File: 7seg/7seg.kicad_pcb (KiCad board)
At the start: 2 copper layers, 58 x 88 mm, 37 parts, among them J1 Conn_01x07, J2 Conn_01x06, J3 Conn_01x07, J4 Conn_01x06

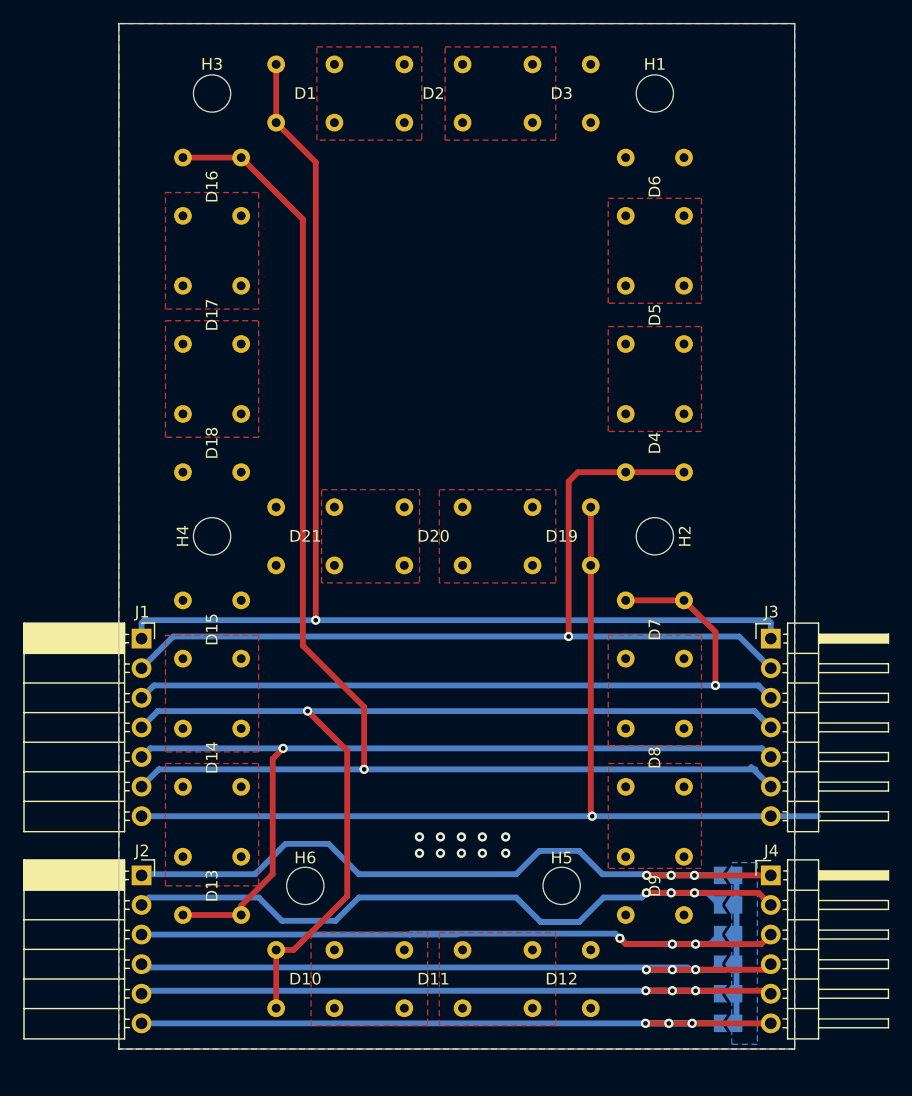
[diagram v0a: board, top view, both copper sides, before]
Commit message: rev 1 of 7seg
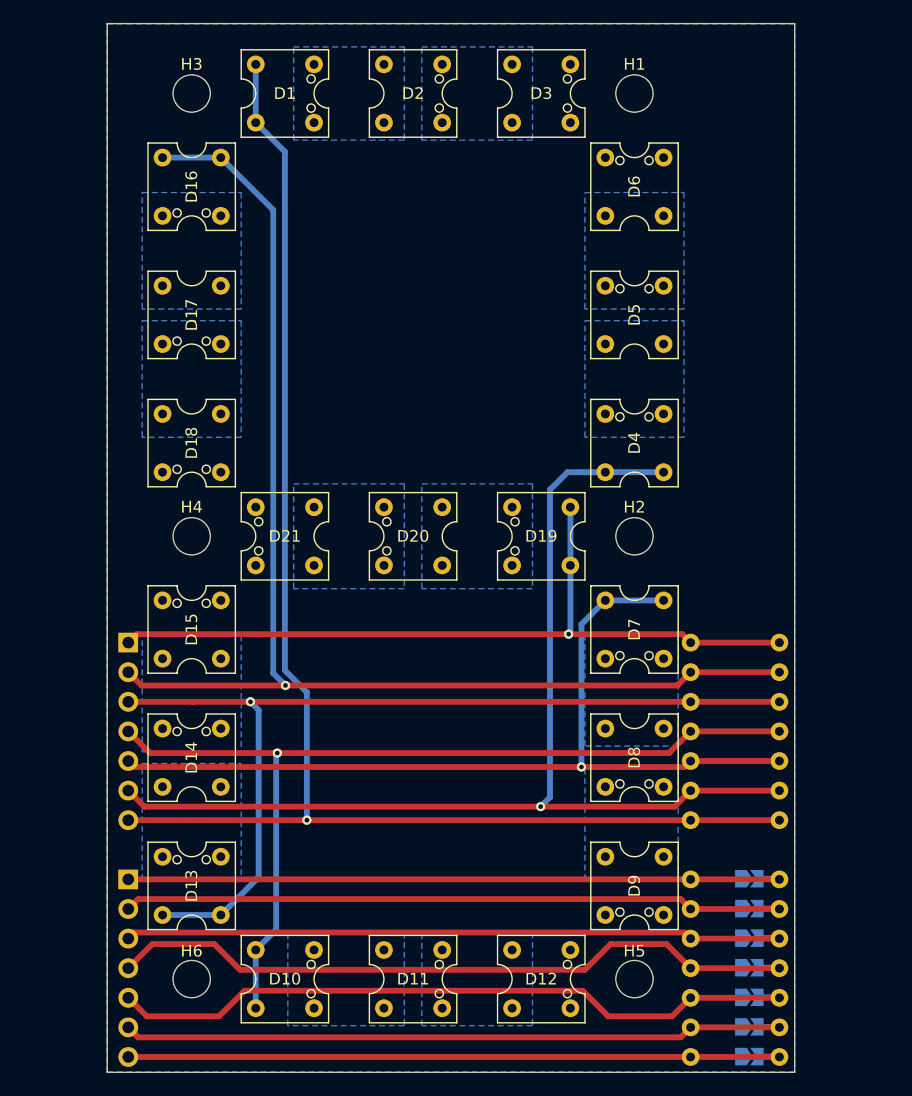
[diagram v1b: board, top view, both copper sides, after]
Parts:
- added JP7: SolderJumper_2_Bridged, Jumper:SolderJumper-2_P1.3mm_Open_TrianglePad1.0x1.5mm, B.Cu at (184.1, 123.4)
- J1: footprint Connector_PinSocket_2.54mm:PinSocket_1x07_P2.54mm_Horizontal -> good_things:pin-socket-7x2.54; moved to B.Cu
- J2: value Conn_01x06 -> Conn_01x07; footprint Connector_PinSocket_2.54mm:PinSocket_1x06_P2.54mm_Horizontal -> good_things:pin-socket-7x2.54; moved to B.Cu
- J3: moved to B.Cu
- J4: value Conn_01x06 -> Conn_01x07; footprint Connector_PinHeader_2.54mm:PinHeader_1x06_P2.54mm_Horizontal -> Connector_PinHeader_2.54mm:PinHeader_1x07_P2.54mm_Horizontal; moved to B.Cu
- moved J3 55.1 mm to (130.8, 103.1), turned to 180 degrees
- moved J4 55.1 mm to (130.8, 123.4), turned to 180 degrees
- moved J1 51.5 mm to (182.9, 110.7), turned to 270 degrees
- moved J2 51.5 mm to (182.9, 131.1), turned to 270 degrees
- moved JP1 15.7 mm to (184.1, 138.6), turned to 0 degrees
- moved H6 12.6 mm to (136.2, 132.0)
- moved JP2 10.6 mm to (184.1, 136.1), turned to 0 degrees
- moved H5 10.2 mm to (174.2, 132.0)
- moved JP6 10.0 mm to (184.1, 125.9), turned to 0 degrees
- moved JP3 5.69 mm to (184.1, 133.6), turned to 0 degrees
- moved JP5 5.11 mm to (184.1, 128.5), turned to 0 degrees
- moved JP4 1.85 mm to (184.1, 131.0), turned to 0 degrees
- moved D1 1.75 mm to (144.2, 56.0)
- moved D10 1.75 mm to (144.2, 132.0)
- moved D11 1.75 mm to (155.2, 132.0)
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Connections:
- J1 pad 1: a -> g
- J1 pad 2: b -> f
- J1 pad 3: c -> e
- J1 pad 5: e -> c
- J1 pad 6: f -> b
- J1 pad 7: g -> a
- J2 pad 1: b0 -> b6
- J2 pad 2: b1 -> b5
- J2 pad 3: b2 -> b4
- J2 pad 5: b4 -> b2
- J2 pad 6: b5 -> b1
- J3 pad 1: a -> g
- J3 pad 2: b -> f
- J3 pad 3: c -> e
- J3 pad 5: e -> c
- J3 pad 6: f -> b
- J3 pad 7: g -> a
- J4 pad 1: b0 -> b6
- J4 pad 2: b1 -> b5
- J4 pad 3: b2 -> b4
- J4 pad 5: b4 -> b2
- J4 pad 6: b5 -> b1
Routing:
- net b6: track 0.00 -> 57.8 mm
- net g: track 84.6 -> 67.4 mm
- net a: track 106.0 -> 122.6 mm
- net b: track 79.8 -> 94.9 mm
- net /com: track 12.7 -> 0.00 mm, vias 10 -> 0
- net c: track 68.3 -> 76.5 mm
- net f: track 117.5 -> 109.4 mm
- net b2: track 67.9 -> 60.9 mm, vias 3 -> 0
- net b0: track 64.7 -> 57.8 mm, vias 3 -> 0
- net b1: track 65.0 -> 58.5 mm, vias 3 -> 0
- net b4: track 64.7 -> 58.2 mm, vias 3 -> 0
- net b5: track 64.4 -> 58.5 mm, vias 3 -> 0
- net e: track 75.4 -> 80.8 mm
- net d: track 85.5 -> 80.6 mm
- net b3: track 64.9 -> 61.3 mm, vias 3 -> 0
- added copper zone on B.Cu, net Net-(D1-Pad1)
- added copper zone on B.Cu, net Net-(D10-Pad1)
- added copper zone on B.Cu, net Net-(D11-Pad1)
- added copper zone on B.Cu, net Net-(D13-Pad1)
- added copper zone on B.Cu, net Net-(D14-Pad1)
- added copper zone on B.Cu, net Net-(D16-Pad1)
- added copper zone on B.Cu, net Net-(D17-Pad1)
- added copper zone on B.Cu, net Net-(D19-Pad1)
- added copper zone on B.Cu, net Net-(D2-Pad1)
- added copper zone on B.Cu, net Net-(D20-Pad1)
- added copper zone on B.Cu, net Net-(D4-Pad1)
- added copper zone on B.Cu, net Net-(D5-Pad1)
- added copper zone on B.Cu, net Net-(D7-Pad1)
- added copper zone on B.Cu, net Net-(D8-Pad1)
- removed copper zone on F.Cu, net Net-(D1-Pad1)
- removed copper zone on F.Cu, net Net-(D10-Pad1)
- removed copper zone on F.Cu, net Net-(D11-Pad1)
- removed copper zone on F.Cu, net Net-(D13-Pad1)
- removed copper zone on F.Cu, net Net-(D14-Pad1)
- removed copper zone on F.Cu, net Net-(D16-Pad1)
- removed copper zone on F.Cu, net Net-(D17-Pad1)
- removed copper zone on F.Cu, net Net-(D19-Pad1)
- removed copper zone on F.Cu, net Net-(D2-Pad1)
- removed copper zone on F.Cu, net Net-(D20-Pad1)
- removed copper zone on F.Cu, net Net-(D4-Pad1)
- removed copper zone on F.Cu, net Net-(D5-Pad1)
- removed copper zone on F.Cu, net Net-(D7-Pad1)
- removed copper zone on F.Cu, net Net-(D8-Pad1)
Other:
- board size 58 x 88 mm -> 59 x 90 mm
- board text added: "Large 7 Segment Display Anton Lööf 2021 Rev 1"
